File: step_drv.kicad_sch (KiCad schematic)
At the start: 63 parts

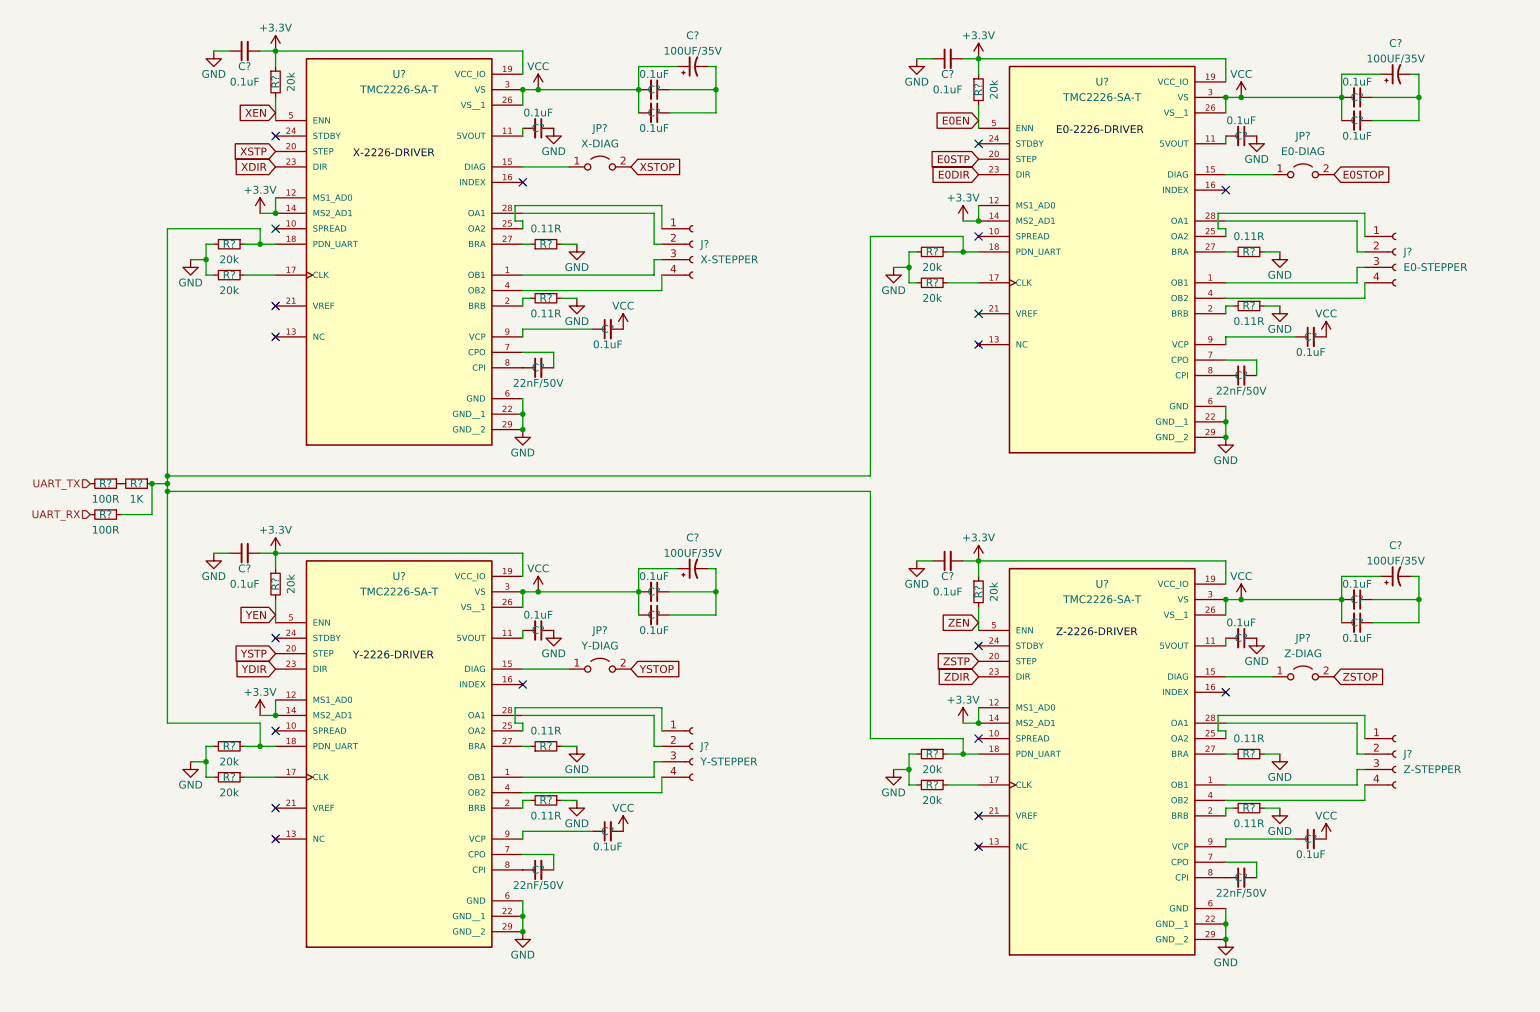
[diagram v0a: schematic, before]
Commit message: Finished Schematic
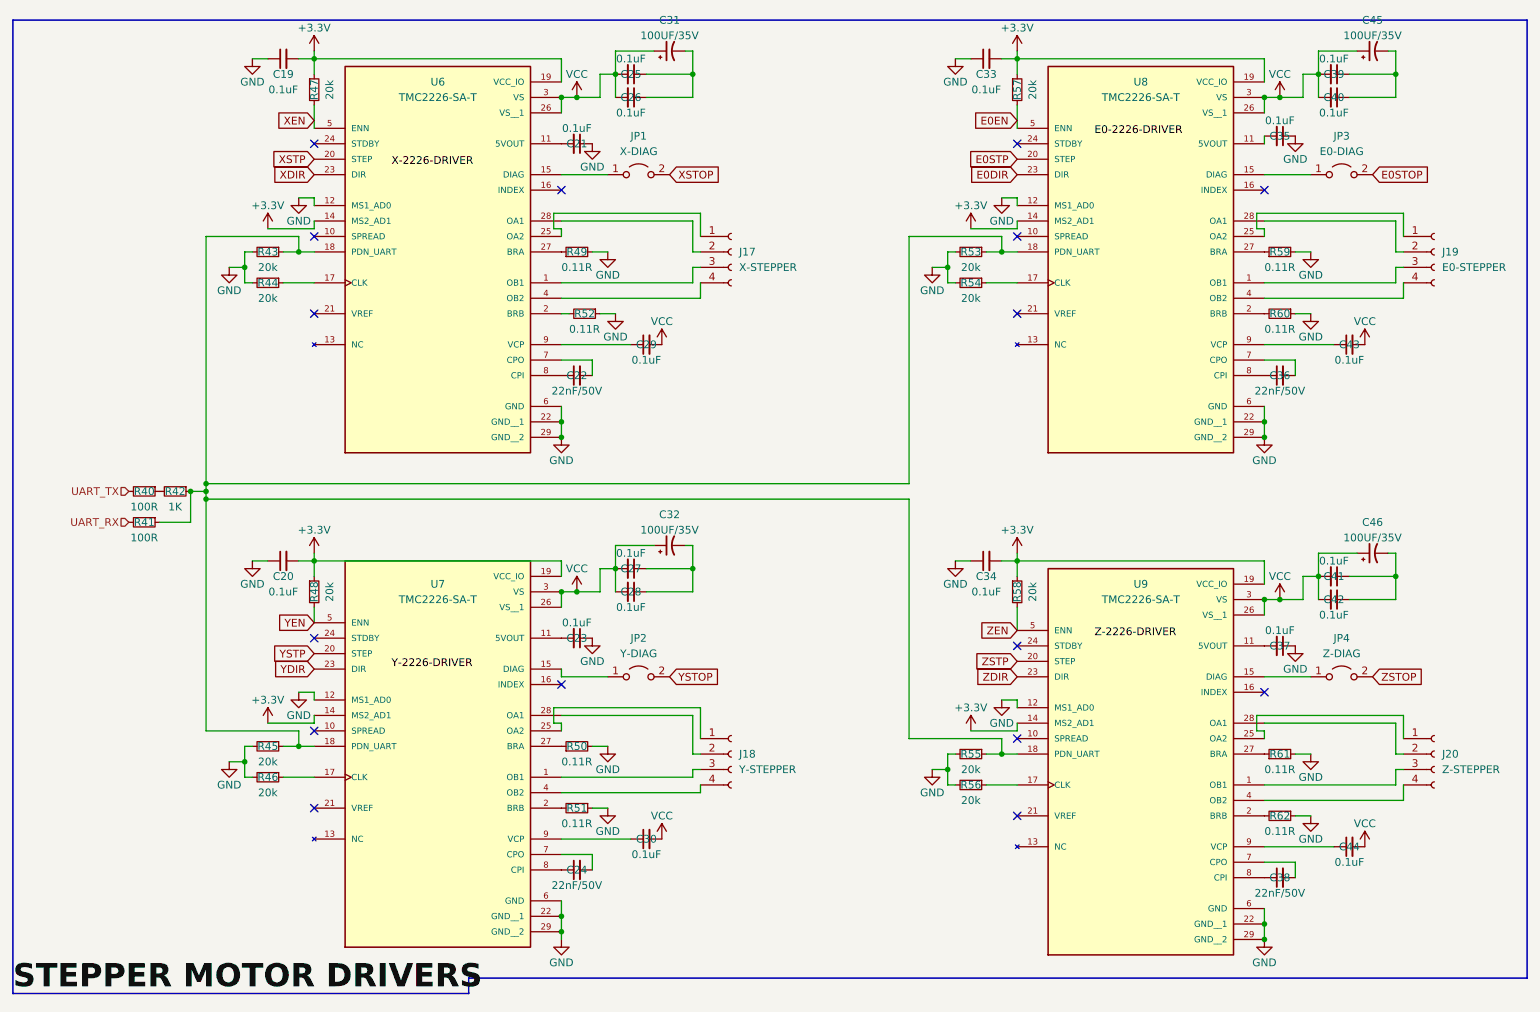
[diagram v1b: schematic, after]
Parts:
- removed C? (x6): 0.1uF, symbol Device:C_Small
- removed C? (x3): 100UF/35V, symbol Device:C_Polarized_Small_US
- added C25, C26, C27, C28, C41, C42: 0.1uF, symbol Device:C_Small
- added C31, C32, C46: 100UF/35V, symbol Device:C_Polarized_Small_US
- gave numbers to parts that had none: 54
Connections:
- net +3.3V: no longer U6.12 (MS1_AD0), U7.12 (MS1_AD0), U8.12 (MS1_AD0), U9.12 (MS1_AD0)
- net GND: now also U6.12 (MS1_AD0), U7.12 (MS1_AD0), U8.12 (MS1_AD0), U9.12 (MS1_AD0)
- net VCC: now also C25.2, C26.2, C27.2, C28.2, C31.1, C32.1, C41.2, C42.2, C46.1
- new net: C25.1, C26.1, C31.2
- new net: C27.1, C28.1, C32.2
- new net: C41.1, C42.1, C46.2
- no-connect marks 20 -> 16
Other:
- moved on the sheet: C19, C20, C21, C22, C23, C24, C29, C30, C33, C34, C35, C36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
